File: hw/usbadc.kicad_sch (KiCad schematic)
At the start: 3 parts, among them J4 JTAG

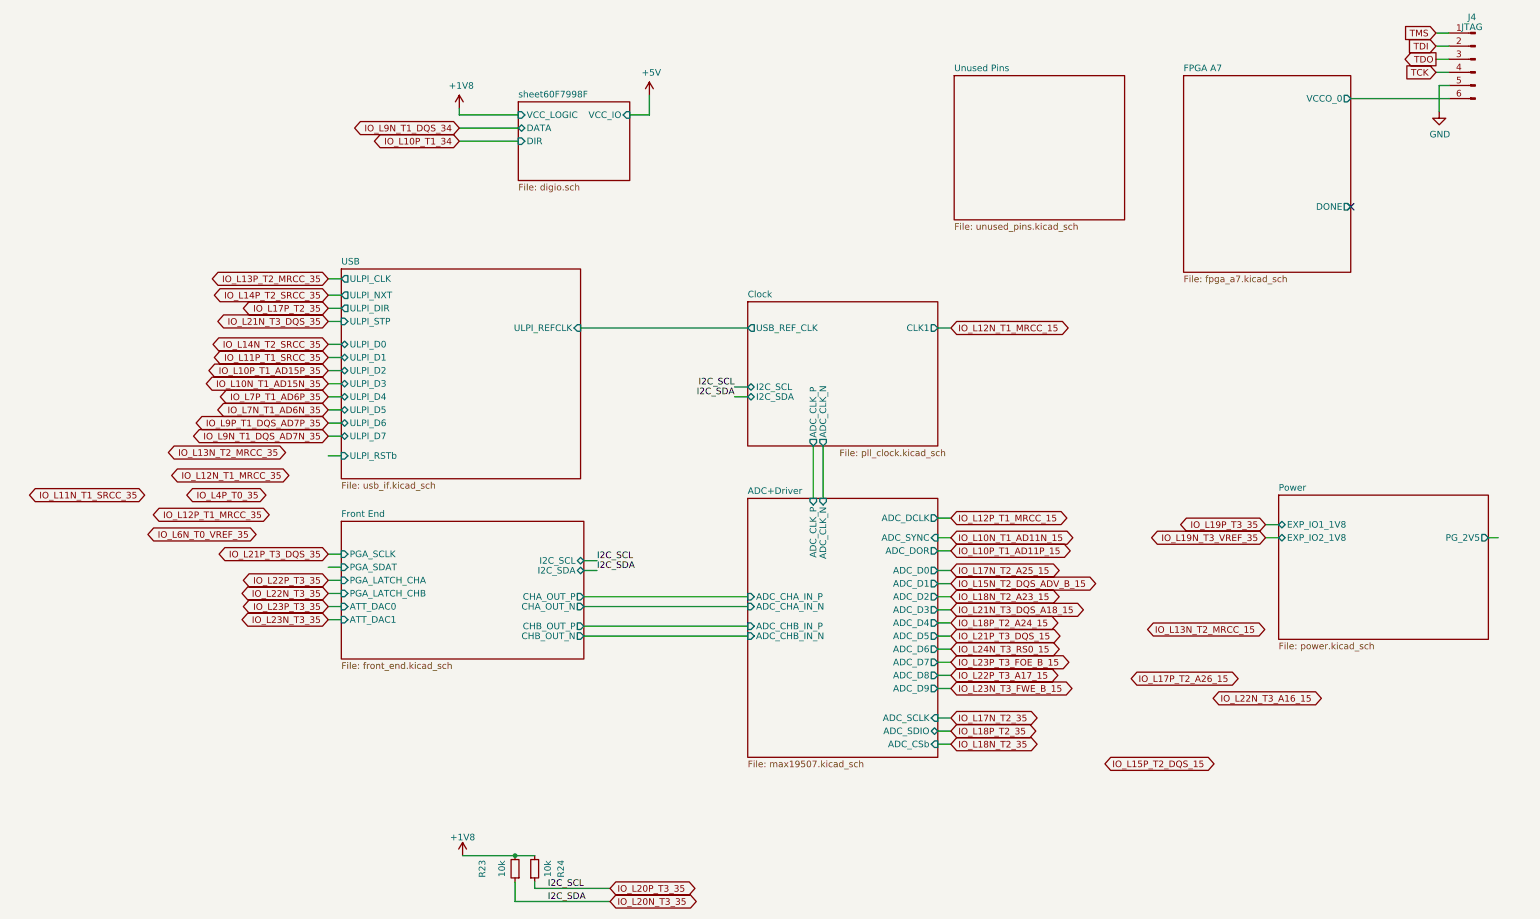
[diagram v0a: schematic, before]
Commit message: WIP - a lot already laid out.
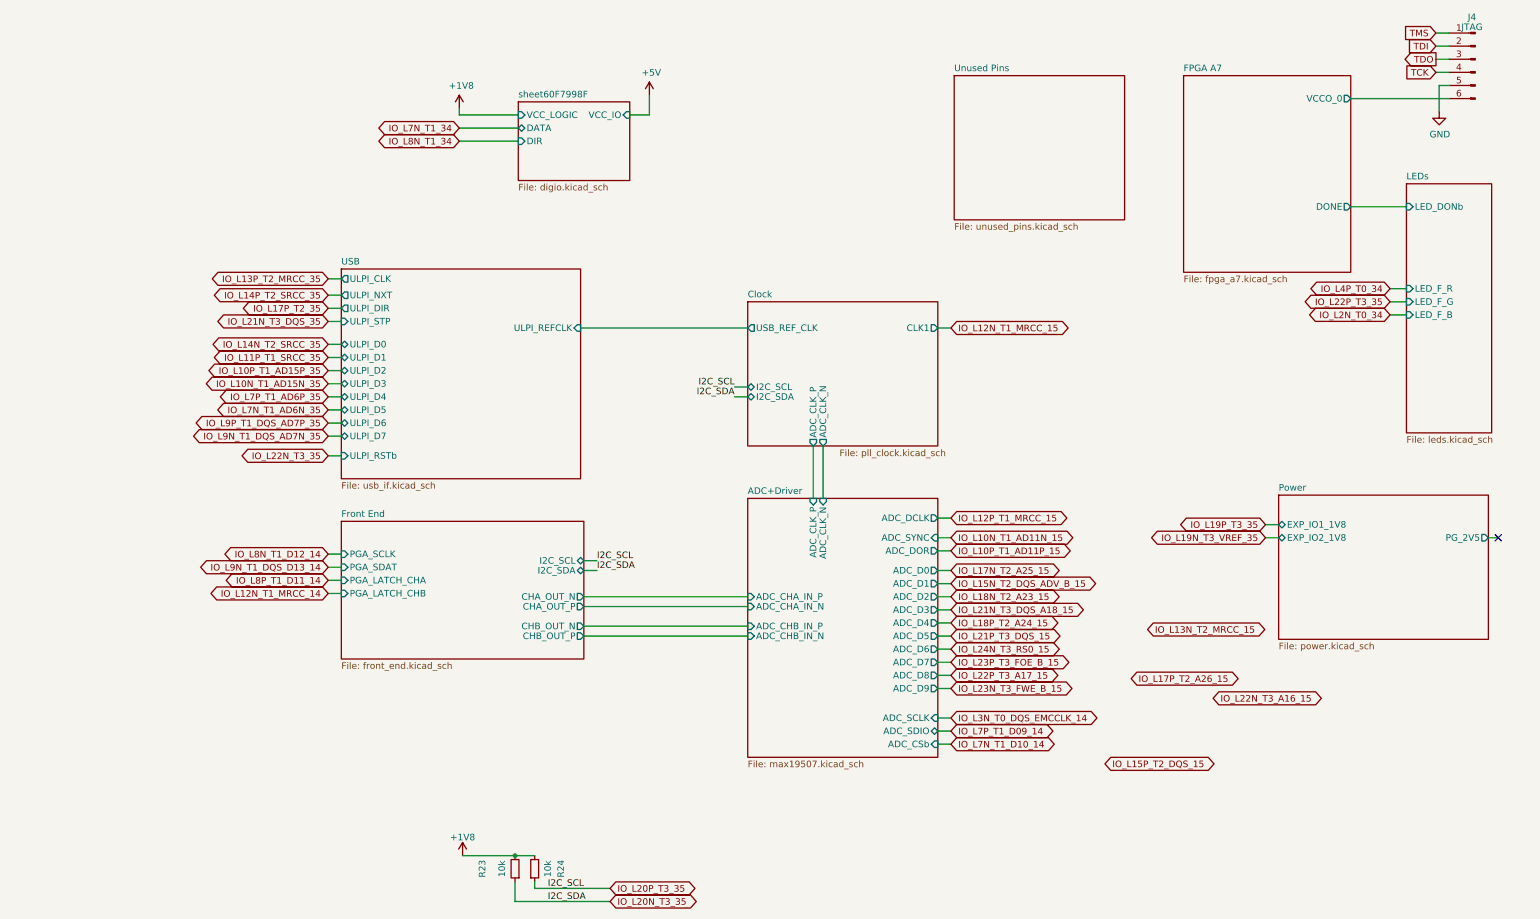
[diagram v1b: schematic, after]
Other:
- added sheet LEDs (leds.kicad_sch)
- sheet Front End ports: added none; removed ATT_DAC0, ATT_DAC1
- sheet sheet60F7998F: file digio.sch -> digio.kicad_sch
